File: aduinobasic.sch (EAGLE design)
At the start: 108 parts, among them SW1 POW

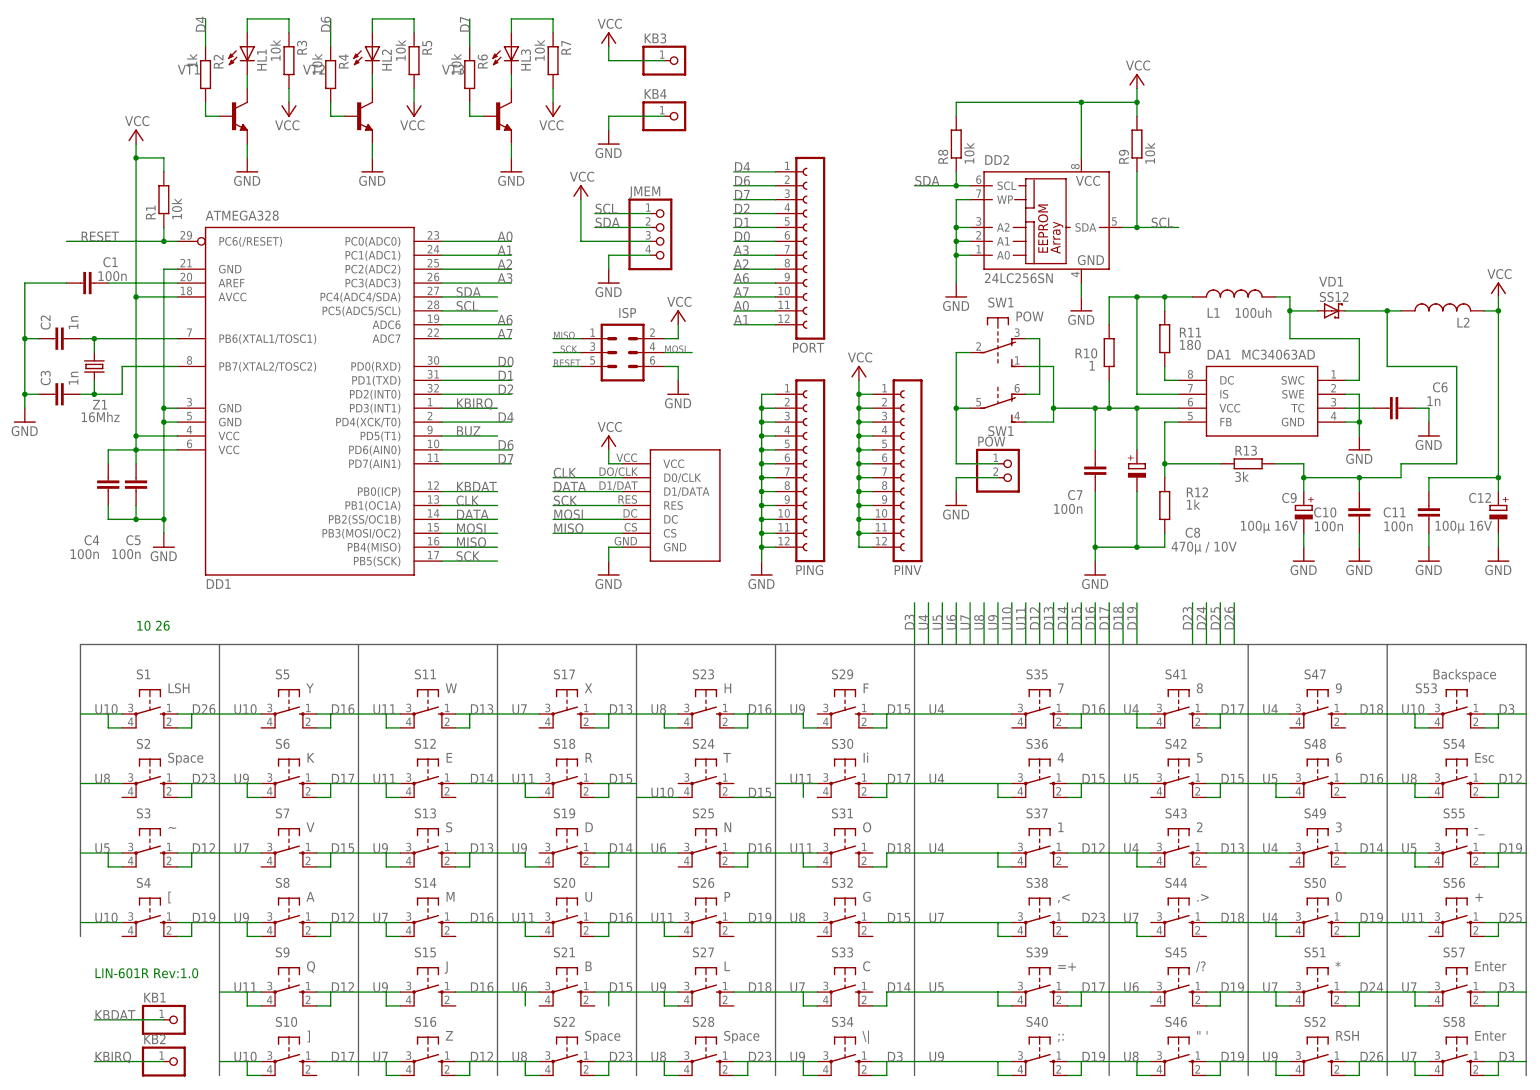
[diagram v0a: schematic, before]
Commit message: .
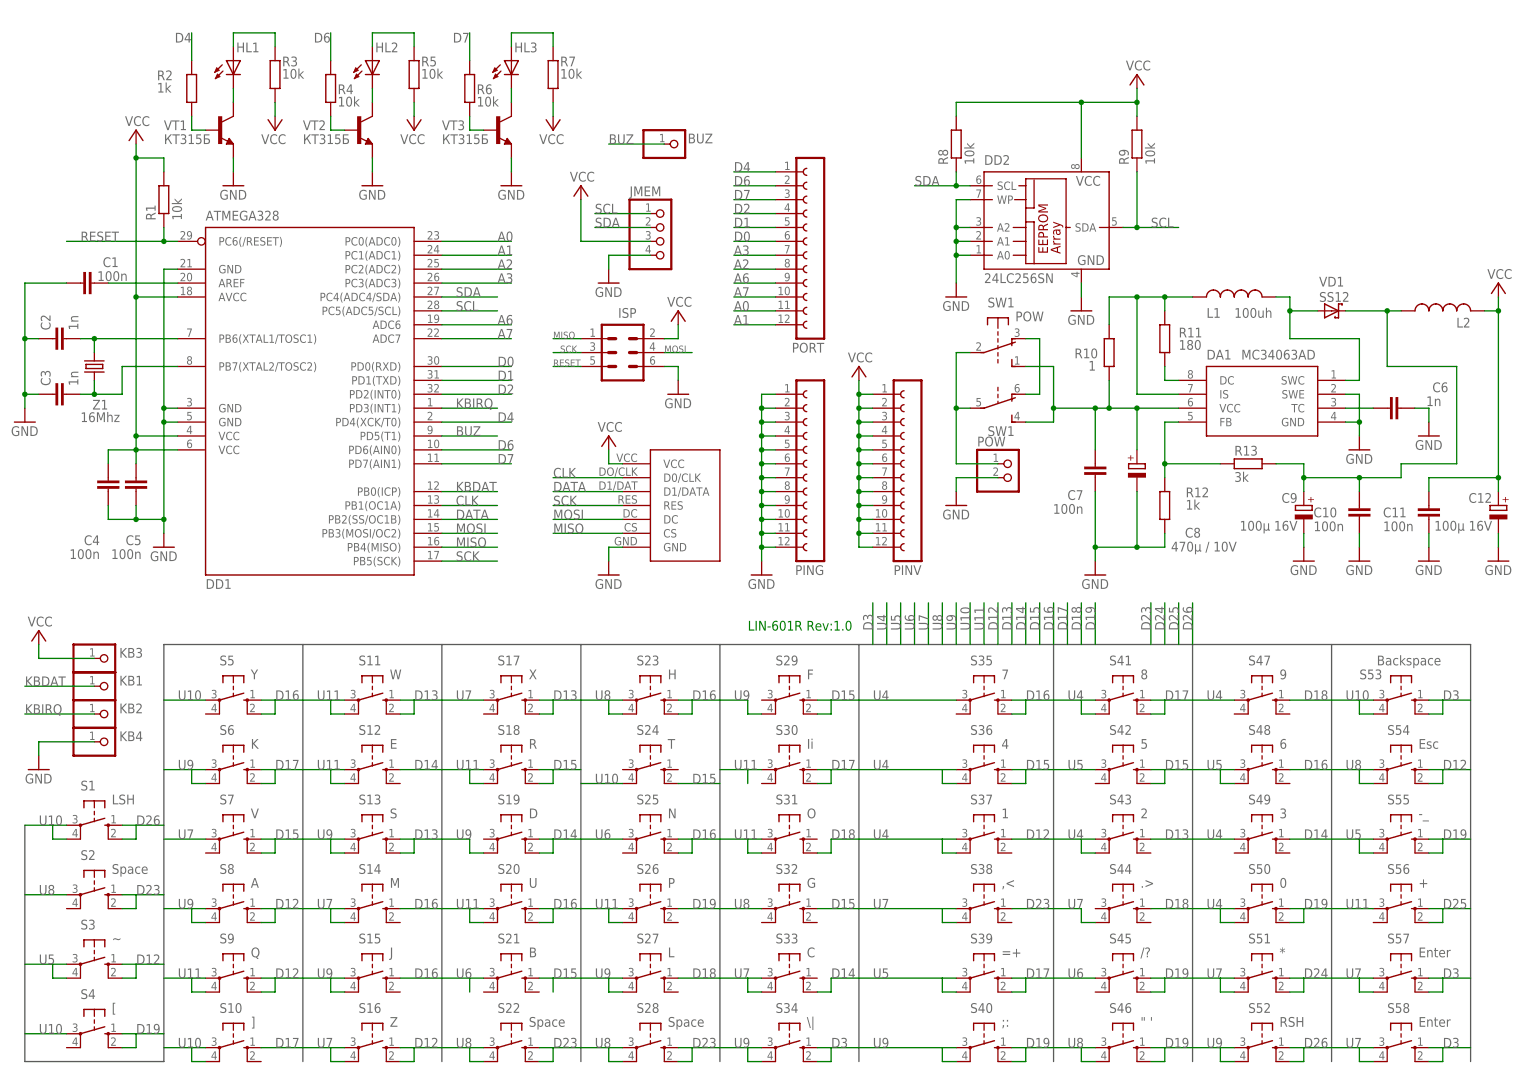
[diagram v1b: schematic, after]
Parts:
- added BUZ: (no value), pinhead:PINHD-1X1
- VT1, VT2, VT3: value (none) -> КТ315Б
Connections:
- net BUZ: now also BUZ.1
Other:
- note removed: "10 26"
- moved on the sheet: HL1, HL2, HL3, KB1, KB2, KB3, KB4, R2, R3, R4, R5, R6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
